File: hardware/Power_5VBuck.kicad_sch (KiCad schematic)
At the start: 12 parts, among them U1 LMR51635XDDCR

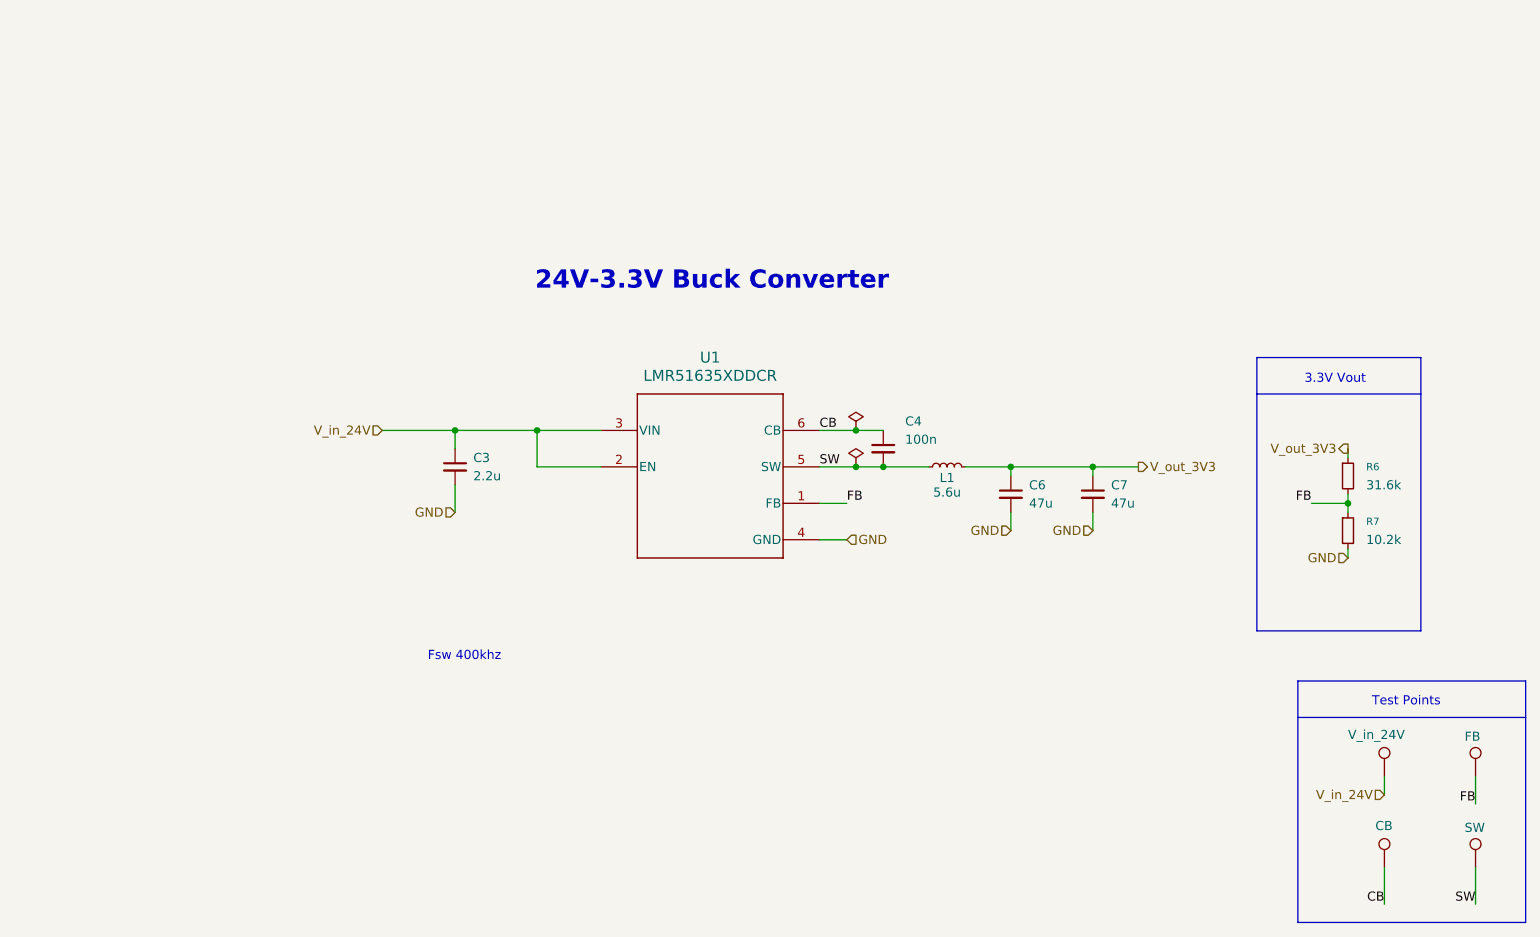
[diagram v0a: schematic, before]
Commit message: power updates
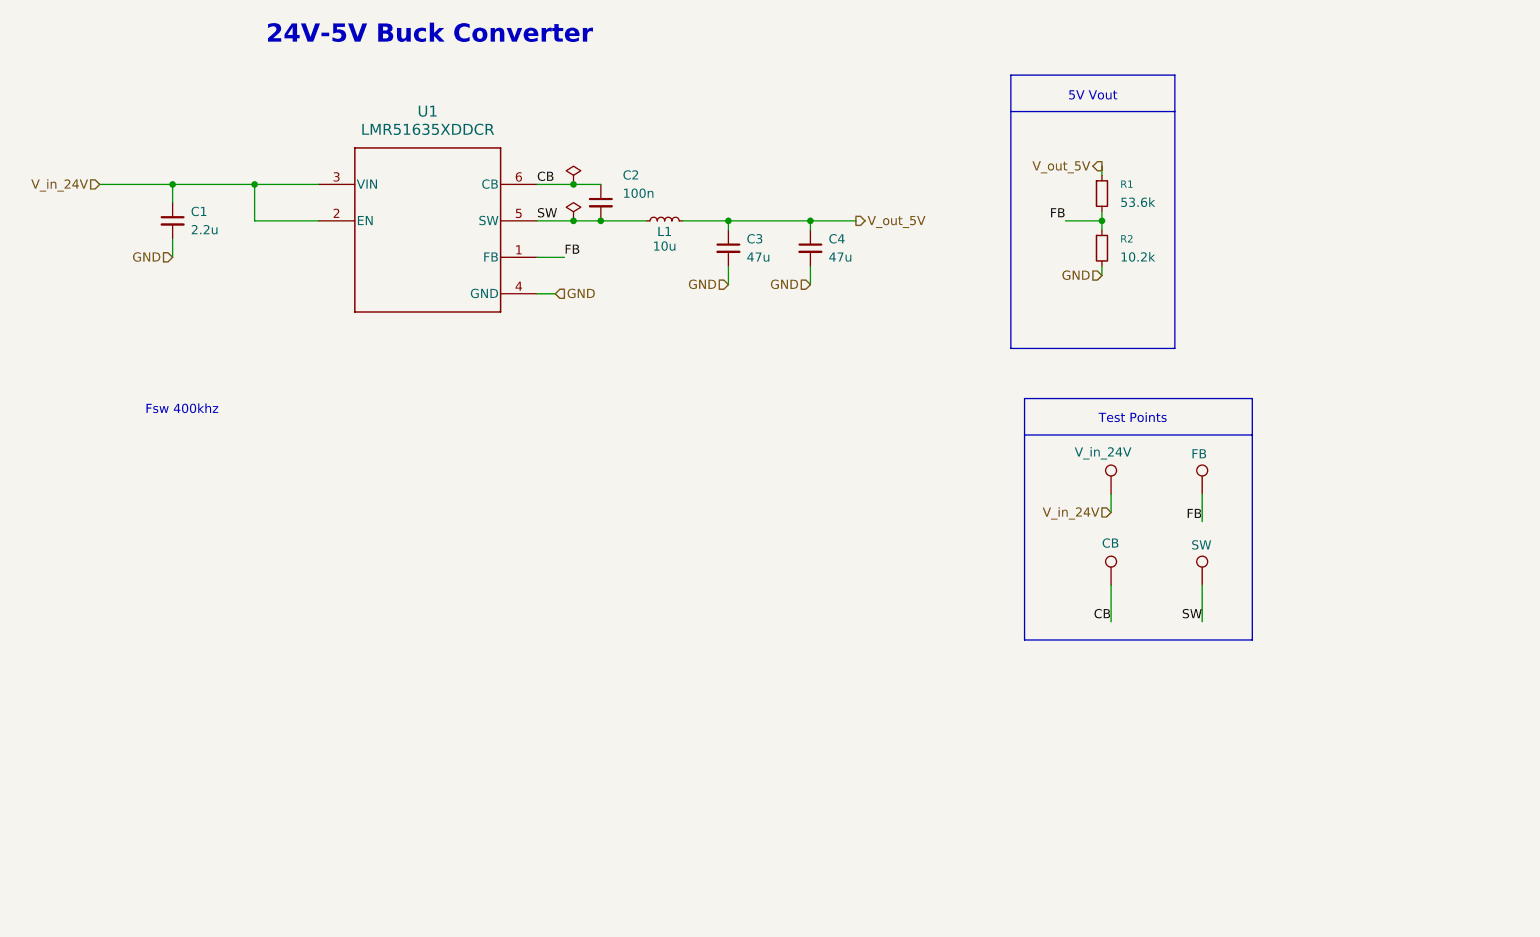
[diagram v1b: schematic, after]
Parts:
- removed C6, C7: 47u, Capacitor_SMD:C_1210_3225Metric_Pad1.33x2.70mm_HandSolder, symbol Device:C_Small
- removed R6: 31.6k, Resistor_SMD:R_0603_1608Metric, symbol Device:R_Small
- removed R7: 10.2k, Resistor_SMD:R_0603_1608Metric, symbol Device:R_Small
- removed TP?: FB, TestPoint:TestPoint_THTPad_D3.0mm_Drill1.5mm, symbol Connector:TestPoint
- removed TP?: SW, TestPoint:TestPoint_THTPad_D3.0mm_Drill1.5mm, symbol Connector:TestPoint
- removed TP?: CB, TestPoint:TestPoint_THTPad_D3.0mm_Drill1.5mm, symbol Connector:TestPoint
- removed TP?: V_in_24V, TestPoint:TestPoint_THTPad_D3.0mm_Drill1.5mm, symbol Connector:TestPoint
- added C1: 2.2u, Capacitor_SMD:C_0805_2012Metric_Pad1.18x1.45mm_HandSolder, symbol Device:C_Small
- added C2: 100n, Capacitor_SMD:C_0603_1608Metric, symbol Device:C_Small
- added R1: 53.6k, Resistor_SMD:R_0603_1608Metric, symbol Device:R_Small
- added R2: 10.2k, Resistor_SMD:R_0603_1608Metric, symbol Device:R_Small
- added TP?: FB, TestPoint:TestPoint_THTPad_D3.0mm_Drill1.5mm, symbol Connector:TestPoint
- added TP?: V_in_24V, TestPoint:TestPoint_THTPad_D3.0mm_Drill1.5mm, symbol Connector:TestPoint
- added TP?: SW, TestPoint:TestPoint_THTPad_D3.0mm_Drill1.5mm, symbol Connector:TestPoint
- added TP?: CB, TestPoint:TestPoint_THTPad_D3.0mm_Drill1.5mm, symbol Connector:TestPoint
- C3: value 2.2u -> 47u; footprint Capacitor_SMD:C_0805_2012Metric_Pad1.18x1.45mm_HandSolder -> Capacitor_SMD:C_1210_3225Metric_Pad1.33x2.70mm_HandSolder; LCSC P/N C1771 -> C77101; P/N CL21F225ZAFNNNE -> GRM32ER61C476KE15L
- C4: value 100n -> 47u; footprint Resistor_SMD:R_0201_0603Metric_Pad0.64x0.40mm_HandSolder -> Capacitor_SMD:C_1210_3225Metric_Pad1.33x2.70mm_HandSolder; LCSC P/N C14663 -> C77101; P/N MLASH168SB7104KTNA01 -> GRM32ER61C476KE15L
- L1: value 5.6u -> 10u; footprint Inductor_SMD:L_TDK_SLF6025 -> LHRS_Passives:SRN8040-101M; LCSC P/N C2997651 -> C54563397; P/N PNLS6045-5R6M 5.6UH -> SRN8040-101M
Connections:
- net CB: now also C2.1, TP?.1; no longer C4.1
- net FB: now also R1.2, R2.1, TP?.1
- net GND: now also C4.2, C1.2, R2.2
- net SW: now also C2.2, TP?.1; no longer C4.2
- net V_in_24V: now also C1.1, TP?.1; no longer C3.1
- net V_out_3V3 renamed V_out_5V
- net V_out_5V: now also C3.1, C4.1, R1.1
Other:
- note added: "24V-5V Buck Converter"
- note added: "5V Vout"
- note removed: "24V-3.3V Buck Converter"
- note removed: "3.3V Vout"
